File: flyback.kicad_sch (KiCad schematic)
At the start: 33 parts, among them Q1 BSC109N10NS3 G, Q2 FQD5N60C, U1 LT3750EMS#PBF, U2 ZXGD3009E6, U3 MCP6V51, U9 MCP4562T-503E/MF

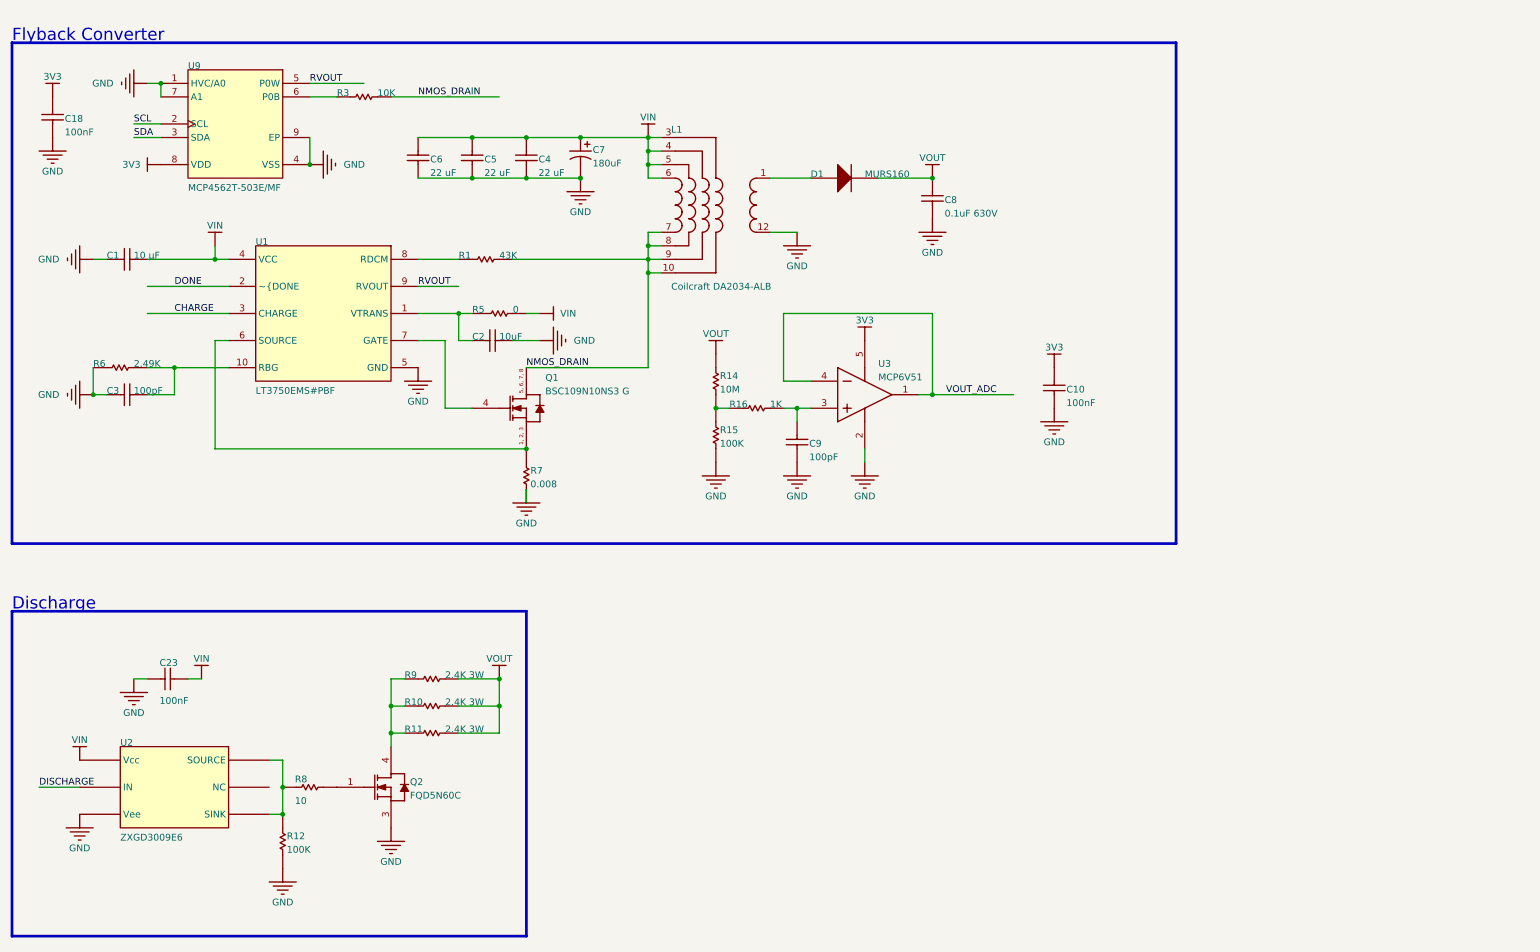
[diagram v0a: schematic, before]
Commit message: Cleanup the project after moving to KiCad.
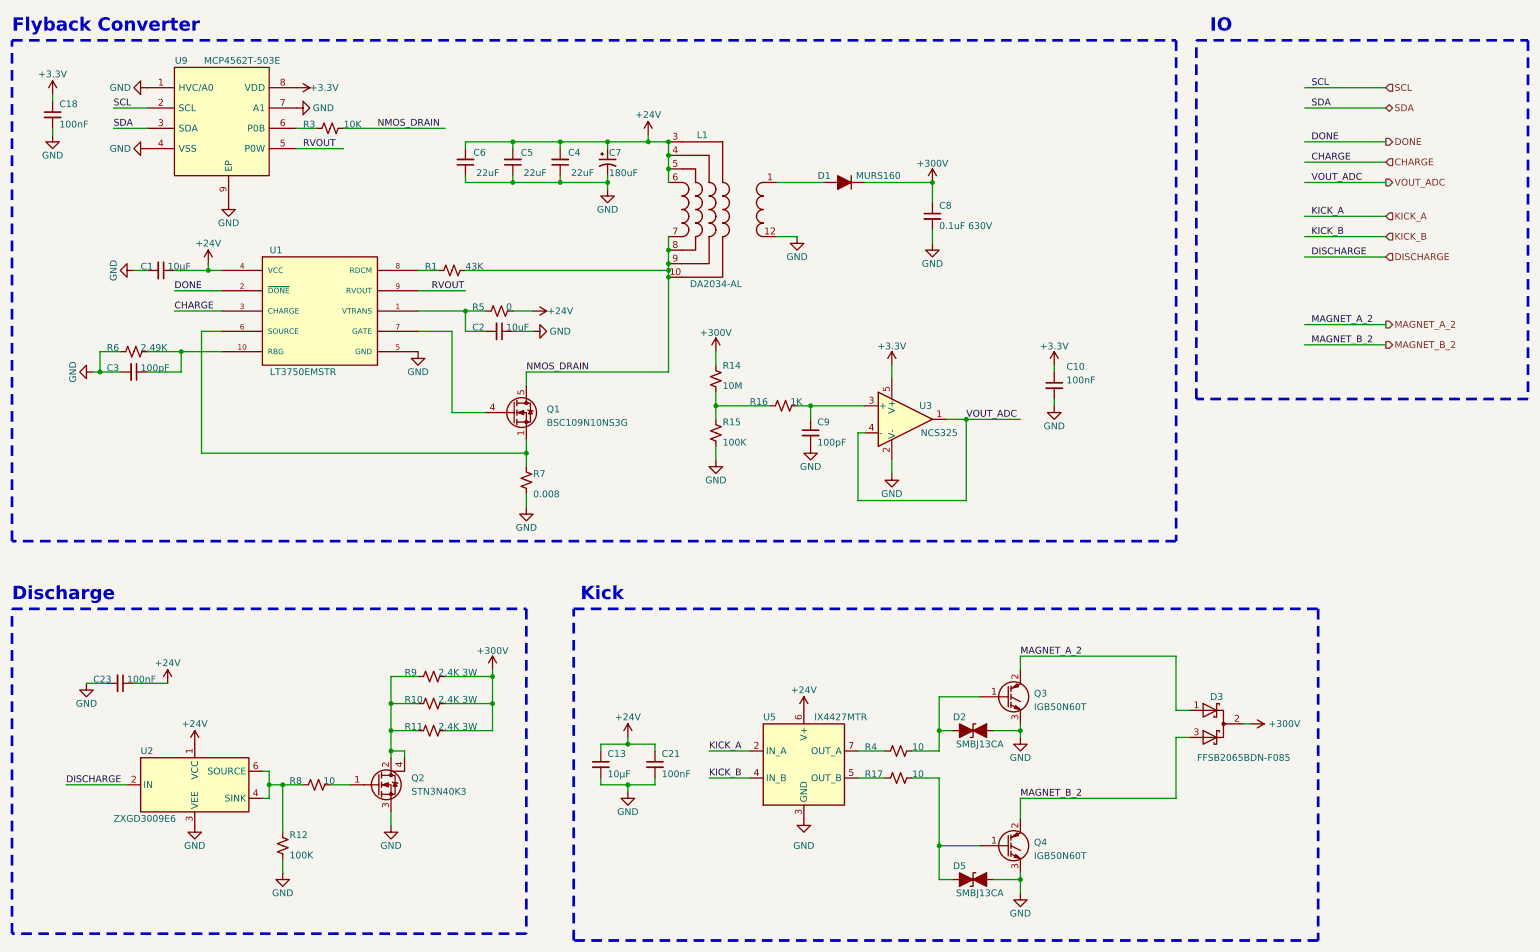
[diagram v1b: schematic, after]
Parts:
- removed D1: MURS160, PCB-1avwftqup47cwryg2qb4-1, symbol mikona-altium-import:0_SYM-7503bc0c42f0aac4-1
- removed L1: Coilcraft DA2034-ALB, LCC18, symbol mikona-altium-import:2_mirrored_SYM-c6870feb3c601940-1
- removed Q1: BSC109N10NS3 G, INF-PG-TDSON-8-1_V, symbol mikona-altium-import:0_INF-NEMOS-SSSGDDDD-8
- removed Q2: FQD5N60C, PCB-yetu4xpugvmduszhgs8y-1, symbol mikona-altium-import:0_SYM-bdc371cf2d746204-1
- removed U1: LT3750EMS#PBF, LT-MS-10_N, symbol mikona-altium-import:0_LT-LT3750-MS-10
- removed U2: ZXGD3009E6, MF06A_N, symbol mikona-altium-import:0_SYM-5e91956982b58156-1
- removed U3: MCP6V51, ADI-RJ-5_L, symbol mikona-altium-import:0_ADI-AD80XX-5
- removed U9: MCP4562T-503E/MF, DFN-MF8, symbol mikona-altium-import:0_IN-DPOT-MCP45X1-9
- added C13: 10µF, Capacitor_SMD:C_0805_2012Metric_Pad1.18x1.45mm_HandSolder, symbol Device:C_Small
- added C21: 100nF, Capacitor_SMD:C_0805_2012Metric_Pad1.18x1.45mm_HandSolder, symbol Device:C_Small
- added D1: MURS160, Diode_SMD:D_SMB_Handsoldering, symbol Device:D_Filled
- added D2, D5: SMBJ13CA, Diode_SMD:D_SMB_Handsoldering, symbol Device:D_TVS_Filled
- added D3: FFSB2065BDN-F085, Package_TO_SOT_SMD:TO-263-2, symbol Device:D_Schottky_Dual_CommonCathode_AKA_Parallel
- added L1: DA2034-AL, DA2034-AL:DA2034-AL, symbol DA2034-AL:DA2034-AL
- added Q1: BSC109N10NS3G, Package_TO_SOT_SMD:TDSON-8-1, symbol Transistor_FET:BSC109N10NS3G
- added Q2: STN3N40K3, Package_TO_SOT_SMD:SOT-223, symbol Device:Q_NMOS_GDSD
- added Q3, Q4: IGB50N60T, Package_TO_SOT_SMD:TO-263-2, symbol Device:Q_NIGBT_GCE
- added R17, R4: 10, Resistor_SMD:R_0402_1005Metric_Pad0.72x0.64mm_HandSolder, symbol Device:R_Small_US
- added U1: LT3750EMSTR, LT3750EMSTR:MSOP-10_MS, symbol LT3750EMSTR:LT3750EMSTR
- added U2: ZXGD3009E6, Package_TO_SOT_SMD:SOT-23-6, symbol Driver_FET:ZXGD3009E6
- added U3: NCS325, Package_TO_SOT_SMD:SOT-23-5, symbol Amplifier_Operational:NCS325
- added U5: IX4427MTR, Package_DFN_QFN:VDFN-8-1EP_2x2mm_P0.5mm_EP0.9x1.7mm, symbol Driver_FET:MIC4427
- added U9: MCP4562T-503E, MCP4562T-503E_MF:SON65P300X300X100-9N-D, symbol MCP4562T-503E_MF:MCP4562T-503E_MF
- C1: value 10 µF -> 10µF; footprint RESC2013X55X40ML15T20 -> Capacitor_SMD:C_0805_2012Metric_Pad1.18x1.45mm_HandSolder; symbol mikona-altium-import:0_SYM-55069f29b9a38ac1-2 -> Device:C_Small
- C10, C18: footprint PCB-ya5qsrmvtd5pjczft90h-1 -> Capacitor_SMD:C_0402_1005Metric_Pad0.74x0.62mm_HandSolder; symbol mikona-altium-import:1_SYM-f7023f833ffb28c5-1 -> Device:C_Small
- C2: footprint PCB-nvrhrmzuvt0gp2xpn124-1 -> Capacitor_SMD:C_1206_3216Metric_Pad1.33x1.80mm_HandSolder; symbol mikona-altium-import:0_SYM-a26f6bc506b57da8-1 -> Device:C_Small
- C23: footprint PCB-cxx7a5qu32qlaf9eltup-1 -> Capacitor_SMD:C_0402_1005Metric_Pad0.74x0.62mm_HandSolder; symbol mikona-altium-import:0_SYM-5f3e94fc157d80f9-1 -> Device:C_Small
- C3: footprint PCB-fmxckod8eunvntzfi285-1 -> Capacitor_SMD:C_0402_1005Metric_Pad0.74x0.62mm_HandSolder; symbol mikona-altium-import:0_SYM-127ed9b197d7cdb9-1 -> Device:C_Small
- C4, C5, C6: value 22 uF -> 22uF; footprint CAPC3225X270X30NL30 -> Capacitor_SMD:C_1210_3225Metric_Pad1.33x2.70mm_HandSolder; symbol mikona-altium-import:1_CAP-NP-2 -> Device:C_Small
- C7: footprint PCBComponent_1 -> Capacitor_SMD:CP_Elec_8x11.9; symbol mikona-altium-import:3_SYM-587e95a52c5187b9-1 -> Device:C_Polarized_Small_US
- C8: footprint PCB-hxcivebo8v2ep67jp7i8-1 -> Capacitor_SMD:C_1812_4532Metric_Pad1.57x3.40mm_HandSolder; symbol mikona-altium-import:1_SYM-cb7c03fa1c0414bb-1 -> Device:C_Small
- C9: footprint PCB-fmxckod8eunvntzfi285-1 -> Capacitor_SMD:C_0402_1005Metric_Pad0.74x0.62mm_HandSolder; symbol mikona-altium-import:1_SYM-127ed9b197d7cdb9-1 -> Device:C_Small
- R1: footprint RESC1005X40X25ML05T05 -> Resistor_SMD:R_0402_1005Metric_Pad0.72x0.64mm_HandSolder; symbol mikona-altium-import:0_RES-2 -> Device:R_Small_US
- R10, R11, R9: footprint Panasonic ERJ-1TNF22R6U-Footprint-1 -> Resistor_SMD:R_2512_6332Metric_Pad1.40x3.35mm_HandSolder; symbol mikona-altium-import:2_RES-2 -> Device:R_Small_US
- R12: footprint RESC1005X40X25ML10T10 -> Resistor_SMD:R_0402_1005Metric_Pad0.72x0.64mm_HandSolder; symbol mikona-altium-import:1_RES-2 -> Device:R_Small_US
- R14: footprint SMD0603GRID25PAD90 -> Resistor_SMD:R_0603_1608Metric_Pad0.98x0.95mm_HandSolder; symbol mikona-altium-import:1_RES-2 -> Device:R_Small_US
- R15: footprint ERJ-PB3B1002V -> Resistor_SMD:R_0603_1608Metric_Pad0.98x0.95mm_HandSolder; symbol mikona-altium-import:1_ERJ-PB3B1003V -> Device:R_Small_US
- R16: footprint CAPC1608X90X35LL15T15 -> Resistor_SMD:R_0603_1608Metric_Pad0.98x0.95mm_HandSolder; symbol mikona-altium-import:0_RES-1k -> Device:R_Small_US
- R3, R6: footprint RESC1005X40X25ML10T10 -> Resistor_SMD:R_0402_1005Metric_Pad0.72x0.64mm_HandSolder; symbol mikona-altium-import:0_RES-2 -> Device:R_Small_US
- R5: footprint RESC1005X40X25ML05T10 -> Resistor_SMD:R_0402_1005Metric_Pad0.72x0.64mm_HandSolder; symbol mikona-altium-import:2_RES-2 -> Device:R_Small_US
- R7: footprint PCB-lktu9k9qvhh1xmnw65nf-1 -> Resistor_SMD:R_0805_2012Metric_Pad1.20x1.40mm_HandSolder; symbol mikona-altium-import:1_SYM-a1d56aab0ef07e12-1 -> Device:R_Small_US
- R8: footprint RESC1005X40X25NL05T05 -> Resistor_SMD:R_0402_1005Metric_Pad0.72x0.64mm_HandSolder; symbol mikona-altium-import:0_RES-2 -> Device:R_Small_US
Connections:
- net 3V3 is gone; now on net GND: C10.2, C18.2
- net CHARGE: now also U1.3 (CHARGE)
- net DISCHARGE: now also U2.2 (IN)
- net DONE: now also U1.2 (~{DONE})
- net GND: now also C1.2, C2.1, C23.2, C3.2, C8.2, C9.2, R12.2, R15.2, R6.2, R7.2, C13.2, C21.2, D2.2 (A2), D5.2 (A2), L1.12, Q2.3 (S), Q3.3 (E), Q4.3 (E), U1.5 (GND), U2.3 (VEE), U3.2 (V-), U5.3 (GND), U9.1 (HVC/A0), U9.4 (VSS), U9.7 (A1), U9.9 (EP); no longer C1.1, C10.1, C18.1, C2.2, C23.1, C3.1, C8.1, C9.1, R12.1, R15.1, R6.1, R7.1
- net NMOS_DRAIN: now also R1.1, R3.1, L1.10, L1.7, L1.8, L1.9, Q1.5 (D); no longer R1.2, R3.2
- net RVOUT: now also U1.9 (RVOUT), U9.5 (P0W)
- net SCL: now also U9.2 (SCL)
- net SDA: now also U9.3 (SDA)
- net VOUT_ADC: now also U3.1, U3.4 (-)
- net at R16.2: now also R14.2, R15.1; no longer C9.2
- net at R8.1: now also Q2.1 (G); no longer R12.2
- net at R10.2, R11.2, R9.2: now also Q2.2 (D), Q2.4 (D)
- net at R8.2: now also R12.1, U2.4 (SINK), U2.6 (SOURCE)
- net at R5.2: now also C2.2, U1.1 (VTRANS); no longer C2.1
- net VIN renamed +24V
- net +24V: now also C1.1, C23.1, C13.1, C21.1, L1.3, L1.4, L1.5, L1.6, U1.4 (VCC), U2.1 (VCC), U5.6 (V+); no longer C1.2, C23.2
- net VOUT renamed +3.3V
- net +3.3V: now also C10.1, C18.1, C8.1, R14.1, D1.1 (K), D3.2 (A), U3.5 (V+), U9.8 (VDD); no longer C8.2, R14.2
- new net: D5.1 (A1), Q4.1 (G), R17.1
- new net: D2.1 (A1), Q3.1 (G), R4.1
- new net: R1.2, U1.8 (RDCM)
- new net: R17.2, U5.5 (OUT_B)
- new net: R3.2, U9.6 (P0B)
- new net: C9.1, R16.1, U3.3 (+)
- new net: R4.2, U5.7 (OUT_A)
- new net: D1.2 (A), L1.1
- new net: Q1.1 (S), Q1.2 (S), Q1.3 (S), R7.1, U1.6 (SOURCE)
- new net: Q1.4 (G), U1.7 (GATE)
- new net: C3.1, R6.1, U1.10 (RBG)
- new net KICK_A: U5.2 (IN_A)
- new net KICK_B: U5.4 (IN_B)
- new net MAGNET_A_2: D3.1 (K), Q3.2 (C)
- new net MAGNET_B_2: D3.3 (K), Q4.2 (C)
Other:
- note added: "IO"
- note added: "Kick"
